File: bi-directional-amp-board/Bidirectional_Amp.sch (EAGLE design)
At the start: 130 parts, among them J1 73415-2061, J10 73415-2061, J11 73415-2061, J12 73415-2061, J2 73415-2061, J3 22-23-2071, J4 73415-2061, J5 73415-2061, J6 73415-2061, J7 73415-2061, J8 73415-2061, J9 22-23-2031, U1 LTC5536, U10 NC7S32M5X, U11 SN74LV1T34DBVR, U2 LTC6994-1, U3 LTC6994-1, U4 QPC1022, U5 NC7S04M5, U6 TQP9111, U7 TQP3M9035, U8 QPC1022, U9 LTC3428EDDPBF

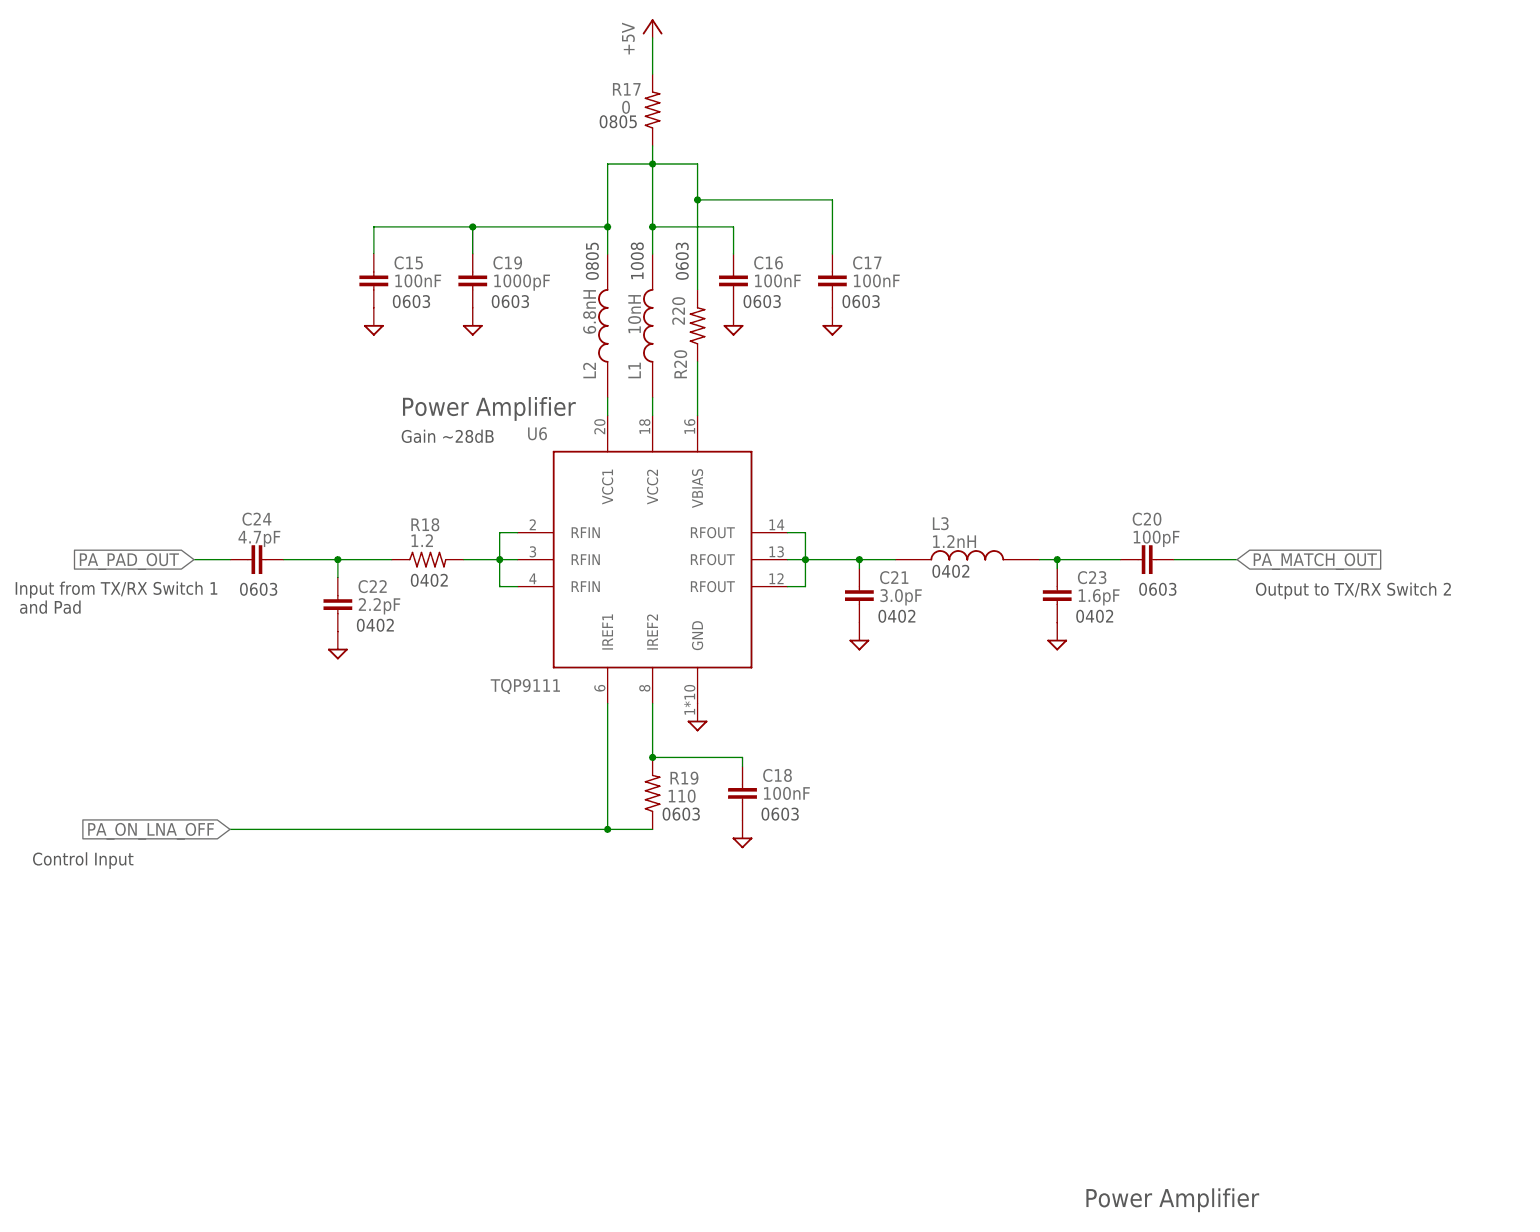
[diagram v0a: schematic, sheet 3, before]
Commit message: still mroe progress on board
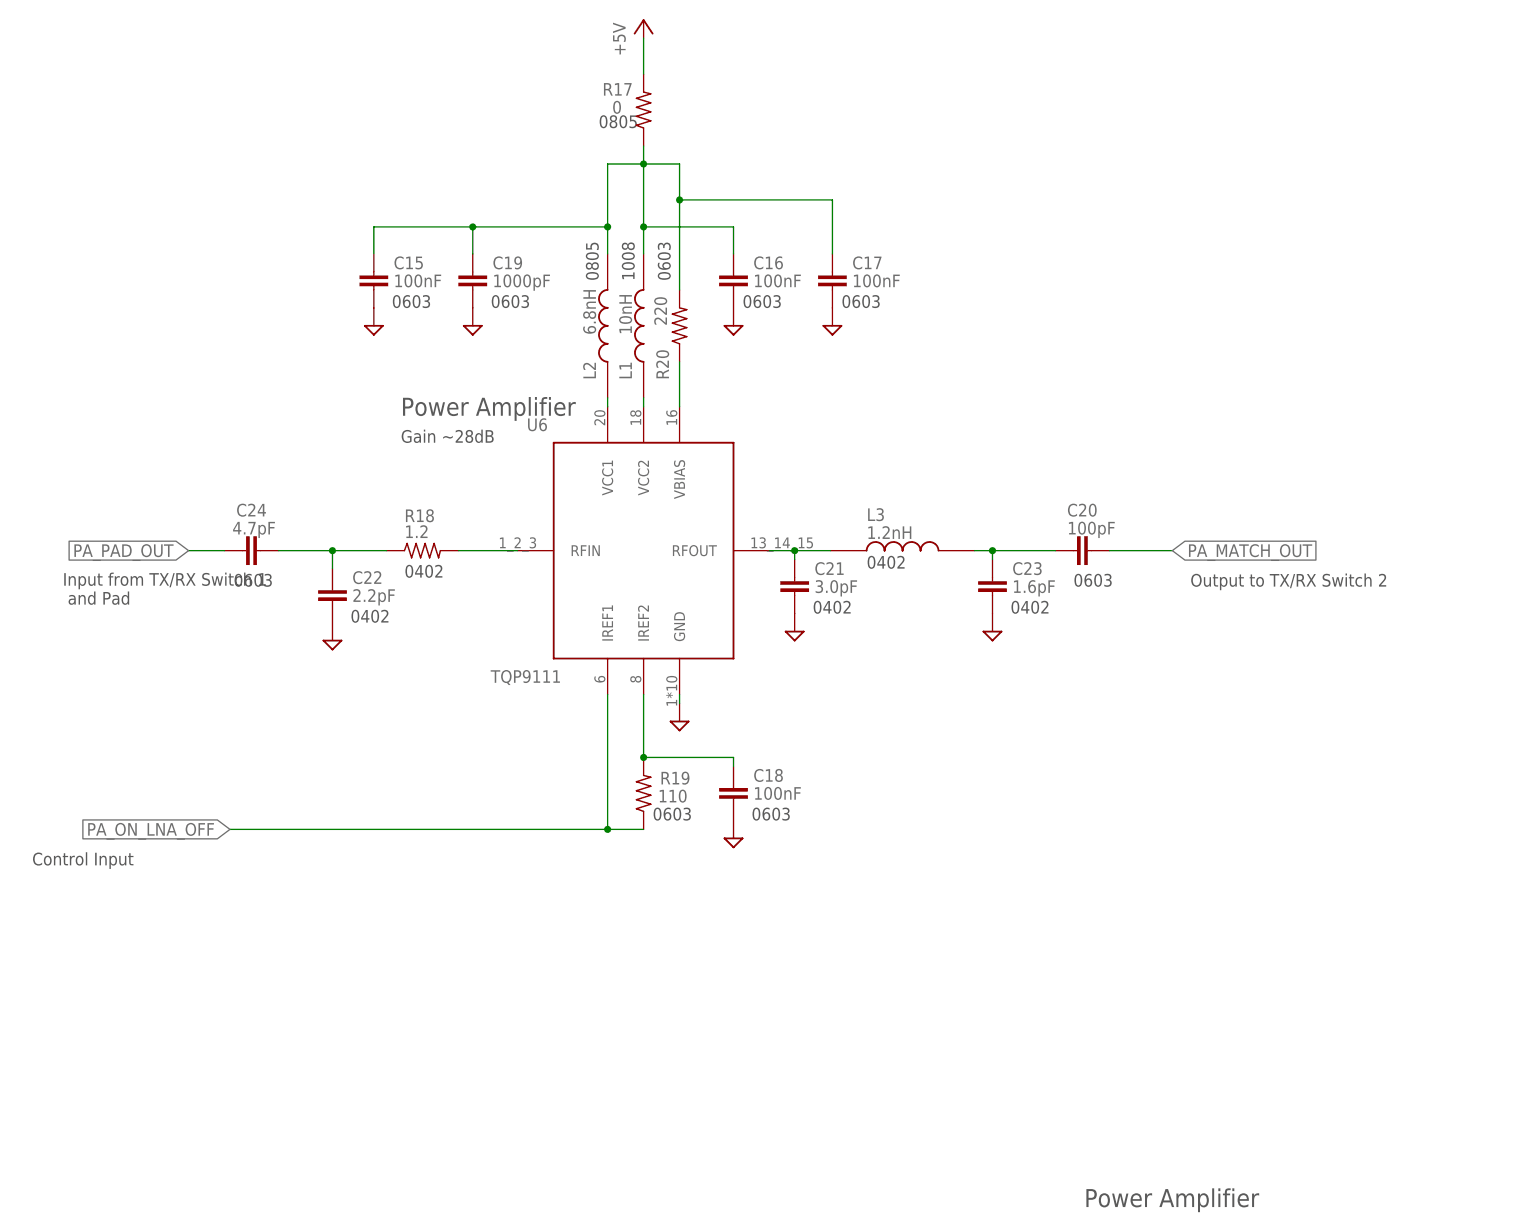
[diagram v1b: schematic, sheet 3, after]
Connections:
- removed net N$23: R18.2, U6.RFIN@2, U6.RFIN@3, U6.RFIN@4
- new net N$56: R18.2, U6.RFIN
- net N$24: now also U6.RFOUT; no longer U6.RFOUT@12, U6.RFOUT@13, U6.RFOUT@14
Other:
- moved on the sheet: C18, C20, C21, C22, C23, C24, L1, L3, R17, R18, R19, R20
